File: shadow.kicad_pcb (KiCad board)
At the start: 2 copper layers, 69.8 x 78.7 mm, 100 parts, among them IC2 XB8089D, J1 USB_C_Receptacle, SW1 SW_Push, SW2 SW_Push, SW3 SW_SPST, U1 TCA9548APWR, U2 TCA9548APWR, U3 BQ24092DGQR, U4 TPS61085DGKR, U5 TPS259621DDAT

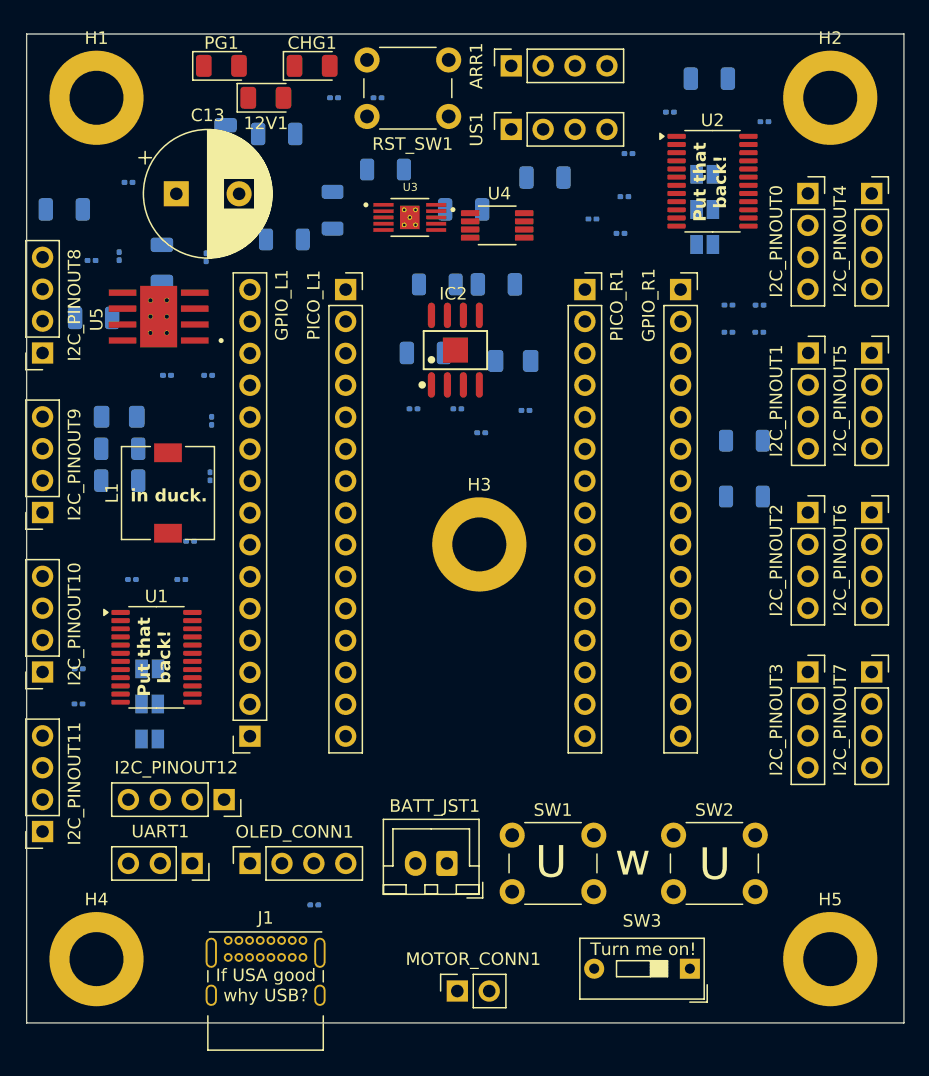
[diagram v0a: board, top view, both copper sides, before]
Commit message: route traces
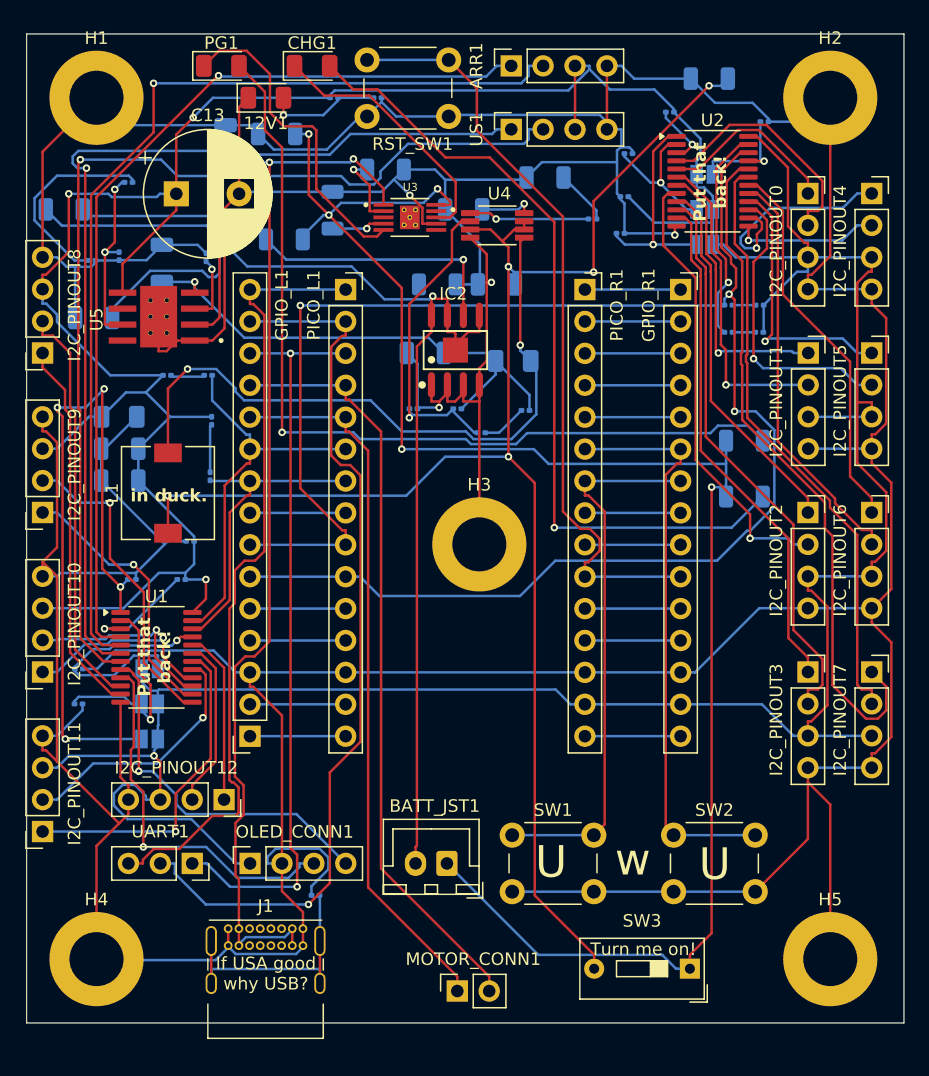
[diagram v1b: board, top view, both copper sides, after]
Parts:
- moved J1 0.94 mm to (114.6, 119.5)
- moved R30 0.77 mm to (121.6, 116.8)
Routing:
- net GND: track 0.00 -> 570.2 mm, vias 0 -> 4
- net VCC: track 0.00 -> 351.8 mm, vias 0 -> 4
- net /battery/BAT+: track 0.00 -> 138.4 mm, vias 0 -> 5
- net Net-(SW3-B): track 0.00 -> 126.4 mm, vias 0 -> 5
- net /battery/BAT-: track 0.00 -> 89.2 mm, vias 0 -> 1
- net Net-(U3-IN): track 0.00 -> 85.8 mm, vias 0 -> 2
- net /US_SCL: track 0.00 -> 82.4 mm, vias 0 -> 1
- net /SENSOR_SCL: track 0.00 -> 80.7 mm, vias 0 -> 1
- net /GPIO9: track 0.00 -> 79.0 mm, vias 0 -> 2
- net /GPIO8: track 0.00 -> 78.9 mm, vias 0 -> 2
- net /US_SDA: track 0.00 -> 78.5 mm, vias 0 -> 1
- net /SENSOR_SDA: track 0.00 -> 74.1 mm, vias 0 -> 1
- net /GPIO1: track 0.00 -> 71.4 mm, vias 0 -> 1
- net Net-(PG1-A): track 0.00 -> 70.4 mm, vias 0 -> 1
- net Net-(CHG1-A): track 0.00 -> 65.0 mm, vias 0 -> 1
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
